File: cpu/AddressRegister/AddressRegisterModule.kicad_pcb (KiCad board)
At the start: 2 copper layers, 100 x 80 mm, 54 parts, among them J1 Bus_PCI_32bit_5V, U1 74LS193, U10 74LS245, U11 74LS245, U12 74LS00, U2 74LS193, U3 74LS193, U4 74LS193, U5 74LS245, U6 74LS245, U7 74LS245, U8 74LS245, U9 74LS245

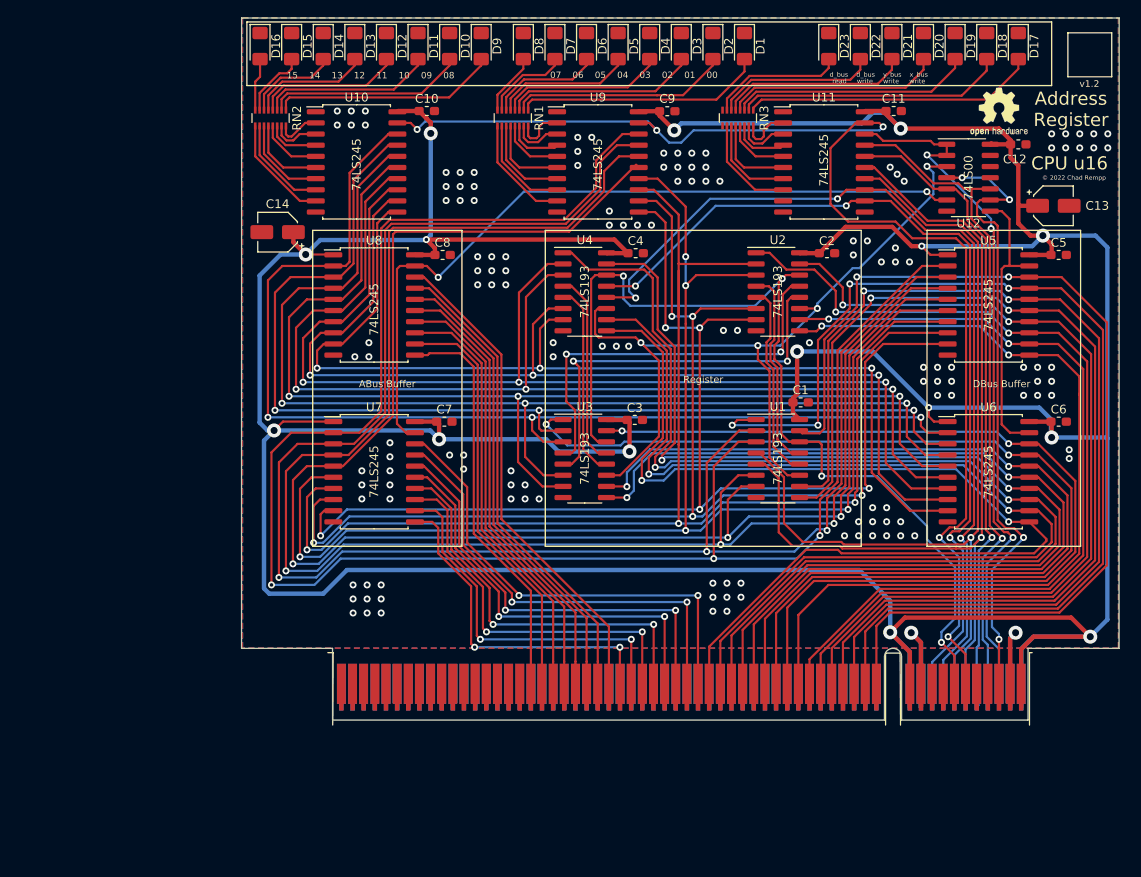
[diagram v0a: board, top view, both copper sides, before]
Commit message: Upgrade to KiCad 6 and commit a bunch of random stuff
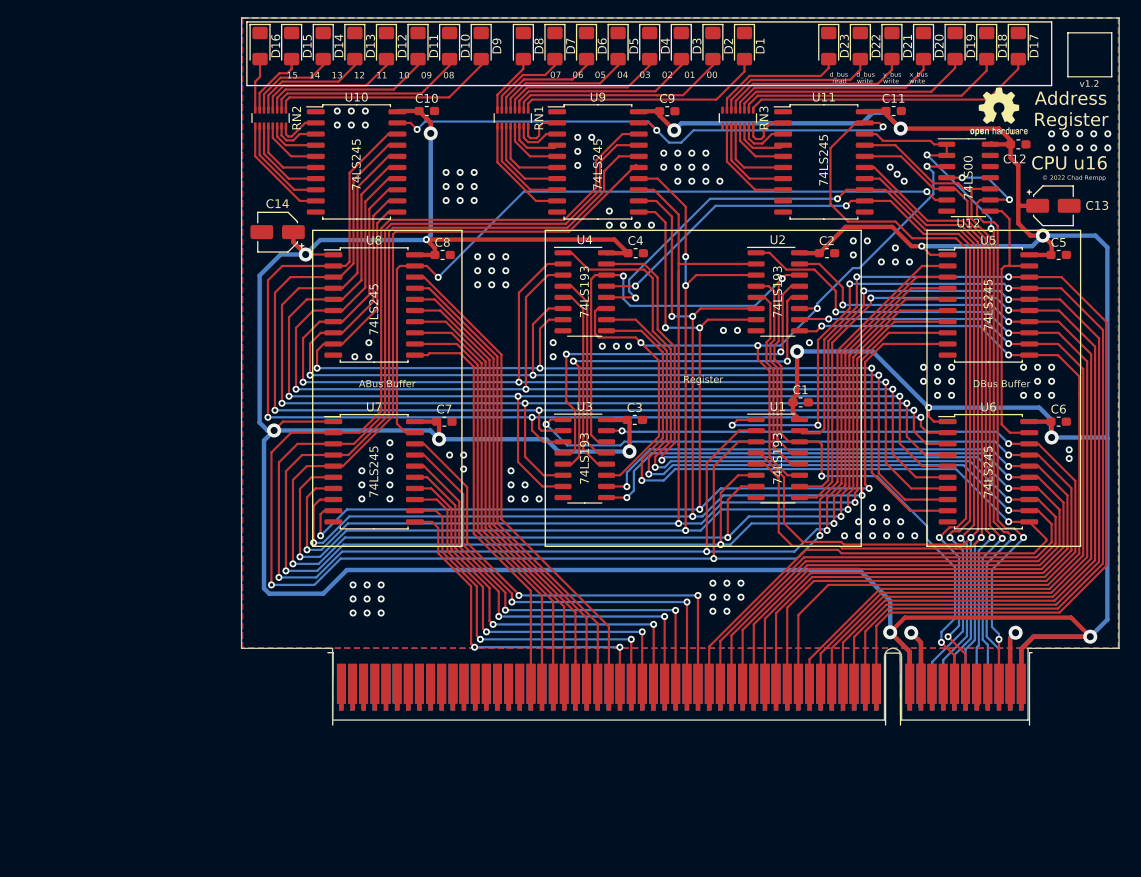
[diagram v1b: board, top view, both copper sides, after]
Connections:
- net /~CLK renamed /~{CLK}
- net /~DBG renamed /~{DBG}
- net /~a_bus_write_CLK renamed /~{a_bus_write_CLK}
- net /~d_bus_read renamed /~{d_bus_read}
- net /~d_bus_write_CLK renamed /~{d_bus_write_CLK}
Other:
- net class Default removed
- net class Power removed

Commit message: Address Register v1.3
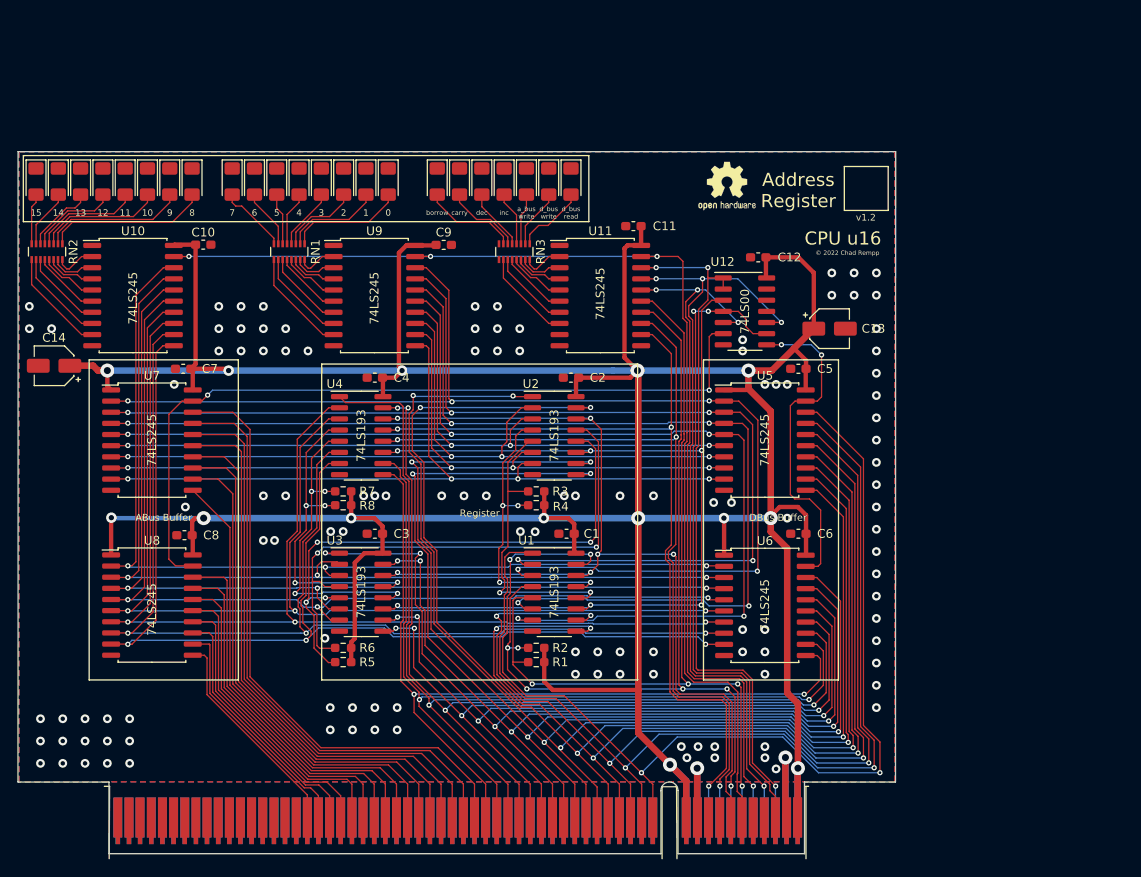
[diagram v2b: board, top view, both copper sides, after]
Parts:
- added R1: 1K, Resistor_SMD:R_0603_1608Metric_Pad0.98x0.95mm_HandSolder, F.Cu at (150.5, 114.2)
- added R2: 1K, Resistor_SMD:R_0603_1608Metric_Pad0.98x0.95mm_HandSolder, F.Cu at (150.5, 112.6)
- added R3: 1K, Resistor_SMD:R_0603_1608Metric_Pad0.98x0.95mm_HandSolder, F.Cu at (150.5, 94.7)
- added R4: 1K, Resistor_SMD:R_0603_1608Metric_Pad0.98x0.95mm_HandSolder, F.Cu at (150.5, 96.3)
- added R5: 1K, Resistor_SMD:R_0603_1608Metric_Pad0.98x0.95mm_HandSolder, F.Cu at (128.5, 114.2)
- added R6: 1K, Resistor_SMD:R_0603_1608Metric_Pad0.98x0.95mm_HandSolder, F.Cu at (128.5, 112.6)
- added R7: 1K, Resistor_SMD:R_0603_1608Metric_Pad0.98x0.95mm_HandSolder, F.Cu at (128.5, 94.7)
- added R8: 1K, Resistor_SMD:R_0603_1608Metric_Pad0.98x0.95mm_HandSolder, F.Cu at (128.5, 96.3)
- C1, C10, C11, C12, C2, C3, C4, C5, C6, C7, C8, C9: value e -> 0.1uF
- moved D17 53.3 mm to (154.4, 59.4)
- moved D18 52.2 mm to (151.9, 59.4)
- moved D19 51.2 mm to (149.4, 59.4)
- moved D20 50.2 mm to (146.8, 59.4)
- moved D21 49.2 mm to (144.3, 59.4)
- moved D22 48.2 mm to (141.7, 59.4)
- moved D23 47.2 mm to (139.2, 59.4)
- moved D1 43.4 mm to (133.6, 59.4)
- moved C8 43.4 mm to (110.4, 99.7), turned to 0 degrees
- moved U8 42.5 mm to (106.7, 107.7)
- moved D2 42.4 mm to (131.1, 59.4)
- moved D3 41.5 mm to (128.5, 59.4)
- moved D4 40.5 mm to (126.0, 59.4)
- moved D5 39.5 mm to (123.4, 59.4)
- moved D6 38.5 mm to (120.9, 59.4)
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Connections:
- J1 pad A1: Net-(J1-PadA1) -> unconnected-(J1-PadA1)
- J1 pad A10: Net-(J1-PadA10) -> unconnected-(J1-PadA10)
- J1 pad A11: Net-(J1-PadA11) -> unconnected-(J1-PadA11)
- J1 pad A12: Net-(J1-PadA12) -> unconnected-(J1-PadA12)
- J1 pad A13: Net-(J1-PadA13) -> unconnected-(J1-PadA13)
- J1 pad A14: Net-(J1-PadA14) -> unconnected-(J1-PadA14)
- J1 pad A15: Net-(J1-PadA15) -> unconnected-(J1-PadA15)
- J1 pad A16: Net-(J1-PadA16) -> unconnected-(J1-PadA16)
- J1 pad A17: Net-(J1-PadA17) -> unconnected-(J1-PadA17)
- J1 pad A18: Net-(J1-PadA18) -> unconnected-(J1-PadA18)
- J1 pad A19: Net-(J1-PadA19) -> unconnected-(J1-PadA19)
- J1 pad A2: Net-(J1-PadA2) -> unconnected-(J1-PadA2)
- J1 pad A20: Net-(J1-PadA20) -> unconnected-(J1-PadA20)
- J1 pad A21: Net-(J1-PadA21) -> unconnected-(J1-PadA21)
- J1 pad A22: Net-(J1-PadA22) -> unconnected-(J1-PadA22)
- J1 pad A23: Net-(J1-PadA23) -> unconnected-(J1-PadA23)
- J1 pad A24: Net-(J1-PadA24) -> unconnected-(J1-PadA24)
- J1 pad A25: Net-(J1-PadA25) -> unconnected-(J1-PadA25)
- J1 pad A26: Net-(J1-PadA26) -> unconnected-(J1-PadA26)
- J1 pad A27: Net-(J1-PadA27) -> unconnected-(J1-PadA27)
- J1 pad A28: Net-(J1-PadA28) -> unconnected-(J1-PadA28)
- J1 pad A29: Net-(J1-PadA29) -> unconnected-(J1-PadA29)
- J1 pad A3: Net-(J1-PadA3) -> unconnected-(J1-PadA3)
- J1 pad A30: Net-(J1-PadA30) -> unconnected-(J1-PadA30)
- J1 pad A31: Net-(J1-PadA31) -> unconnected-(J1-PadA31)
- J1 pad A32: Net-(J1-PadA32) -> unconnected-(J1-PadA32)
- J1 pad A33: Net-(J1-PadA33) -> unconnected-(J1-PadA33)
- J1 pad A34: Net-(J1-PadA34) -> unconnected-(J1-PadA34)
- J1 pad A35: Net-(J1-PadA35) -> unconnected-(J1-PadA35)
- J1 pad A36: Net-(J1-PadA36) -> unconnected-(J1-PadA36)
- J1 pad A37: Net-(J1-PadA37) -> unconnected-(J1-PadA37)
- J1 pad A38: Net-(J1-PadA38) -> unconnected-(J1-PadA38)
- J1 pad A39: Net-(J1-PadA39) -> unconnected-(J1-PadA39)
- J1 pad A4: Net-(J1-PadA4) -> unconnected-(J1-PadA4)
- J1 pad A40: Net-(J1-PadA40) -> unconnected-(J1-PadA40)
- J1 pad A41: Net-(J1-PadA41) -> unconnected-(J1-PadA41)
- J1 pad A42: Net-(J1-PadA42) -> unconnected-(J1-PadA42)
- J1 pad A43: Net-(J1-PadA43) -> unconnected-(J1-PadA43)
- J1 pad A44: Net-(J1-PadA44) -> unconnected-(J1-PadA44)
- J1 pad A45: Net-(J1-PadA45) -> unconnected-(J1-PadA45)
- J1 pad A46: Net-(J1-PadA46) -> unconnected-(J1-PadA46)
- J1 pad A47: Net-(J1-PadA47) -> unconnected-(J1-PadA47)
- J1 pad A48: Net-(J1-PadA48) -> unconnected-(J1-PadA48)
- J1 pad A49: Net-(J1-PadA49) -> unconnected-(J1-PadA49)
- J1 pad A5: Net-(J1-PadA5) -> unconnected-(J1-PadA5)
- J1 pad A6: Net-(J1-PadA6) -> unconnected-(J1-PadA6)
- J1 pad A7: Net-(J1-PadA7) -> unconnected-(J1-PadA7)
- J1 pad A8: Net-(J1-PadA8) -> unconnected-(J1-PadA8)
- J1 pad A9: Net-(J1-PadA9) -> unconnected-(J1-PadA9)
- J1 pad B1: Net-(J1-PadB1) -> unconnected-(J1-PadB1)
- J1 pad B10: Net-(J1-PadB10) -> unconnected-(J1-PadB10)
- J1 pad B11: Net-(J1-PadB11) -> unconnected-(J1-PadB11)
- J1 pad B12: Net-(J1-PadB12) -> unconnected-(J1-PadB12)
- J1 pad B13: Net-(J1-PadB13) -> unconnected-(J1-PadB13)
- J1 pad B14: Net-(J1-PadB14) -> unconnected-(J1-PadB14)
- J1 pad B15: Net-(J1-PadB15) -> unconnected-(J1-PadB15)
- J1 pad B16: Net-(J1-PadB16) -> unconnected-(J1-PadB16)
- J1 pad B17: Net-(J1-PadB17) -> unconnected-(J1-PadB17)
- J1 pad B2: Net-(J1-PadB2) -> unconnected-(J1-PadB2)
- J1 pad B3: Net-(J1-PadB3) -> unconnected-(J1-PadB3)
- J1 pad B4: Net-(J1-PadB4) -> unconnected-(J1-PadB4)
- J1 pad B5: Net-(J1-PadB5) -> unconnected-(J1-PadB5)
- J1 pad B54: Net-(J1-PadB54) -> unconnected-(J1-PadB54)
- J1 pad B55: Net-(J1-PadB55) -> unconnected-(J1-PadB55)
- J1 pad B58: /HLT -> unconnected-(J1-PadB58)
- J1 pad B59: /~{CLK} -> unconnected-(J1-PadB59)
- J1 pad B6: Net-(J1-PadB6) -> unconnected-(J1-PadB6)
- J1 pad B7: Net-(J1-PadB7) -> unconnected-(J1-PadB7)
- J1 pad B8: Net-(J1-PadB8) -> unconnected-(J1-PadB8)
- J1 pad B9: Net-(J1-PadB9) -> unconnected-(J1-PadB9)
- RN3 pad 8: Net-(RN3-Pad8) -> unconnected-(RN3-Pad8)
- RN3 pad 9: Net-(RN3-Pad9) -> unconnected-(RN3-Pad9)
- U11 pad 11: Net-(U11-Pad11) -> unconnected-(U11-Pad11)
- U11 pad 9: Net-(U11-Pad9) -> unconnected-(U11-Pad9)
- U12 pad 11: Net-(U12-Pad11) -> unconnected-(U12-Pad11)
- U12 pad 12: Net-(U12-Pad12) -> unconnected-(U12-Pad12)
- U12 pad 13: Net-(U12-Pad13) -> unconnected-(U12-Pad13)
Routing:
- net +5V: track 540.7 -> 455.0 mm, vias 15 -> 14
- net /reg_01: track 202.9 -> 135.7 mm, vias 3 -> 5
- net /reg_04: track 159.4 -> 92.3 mm, vias 5 -> 4
- net /reg_00: track 205.8 -> 139.3 mm, vias 3 -> 5
- net /reg_05: track 157.7 -> 95.3 mm, vias 3 -> 4
- net /reg_06: track 146.7 -> 90.9 mm, vias 5 -> 4
- net /reg_02: track 190.1 -> 139.5 mm, vias 3 -> 5
- net /reg_07: track 140.6 -> 90.7 mm, vias 5 -> 4
- net /d_bus_04: track 102.5 -> 149.6 mm, vias 2 -> 4
- net /reg_03: track 182.2 -> 138.2 mm, vias 3 -> 5
- net /d_bus_06: track 97.5 -> 140.4 mm, vias 2 -> 4
- net /d_bus_07: track 100.3 -> 137.3 mm, vias 2 -> 4
- net /d_bus_05: track 107.6 -> 141.4 mm, vias 2 -> 4
- net /d_bus_15: track 123.8 -> 96.1 mm
- net /a_bus_15: track 51.0 -> 24.7 mm
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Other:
- board text added: "0"
- board text added: "1"
- board text added: "10"
- board text added: "11"
- board text added: "12"
- board text added: "13"
- board text added: "14"
- board text added: "15"
- board text added: "2"
- board text added: "3"
- board text added: "4"
- board text added: "5"
- board text added: "6"
- board text added: "7"
- board text added: "8"
- board text added: "9"
- board text added: "a_bus write"
- board text added: "borrow"
- board text added: "carry"
- board text added: "d_bus read"
- board text added: "d_bus write"
- board text added: "dec"
- board text added: "inc"
- board text removed: "07 06 05 04 03 02 01 00"
- board text removed: "15 14 13 12 11 10 09 08"
- board text removed: "d_bus d_bus y_bus x_bus"
- board text removed: "read write write write"
